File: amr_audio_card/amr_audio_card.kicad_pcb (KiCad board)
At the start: 2 copper layers, 68.8 x 106.7 mm, 3 parts, among them J1 Conn_Coaxial, J2 USB_A, U1 Bus_AMR

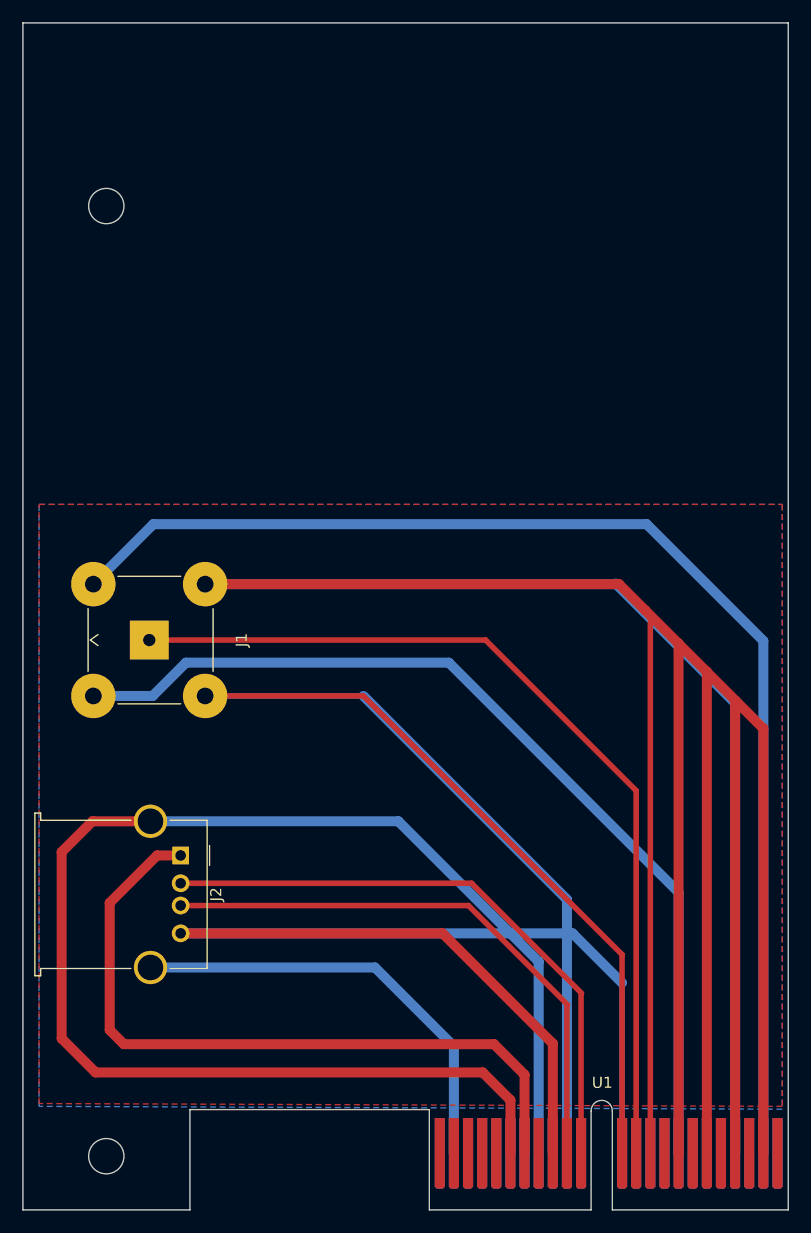
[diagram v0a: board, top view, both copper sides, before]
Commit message: yeah i don't need a bunch of empty space fabricated
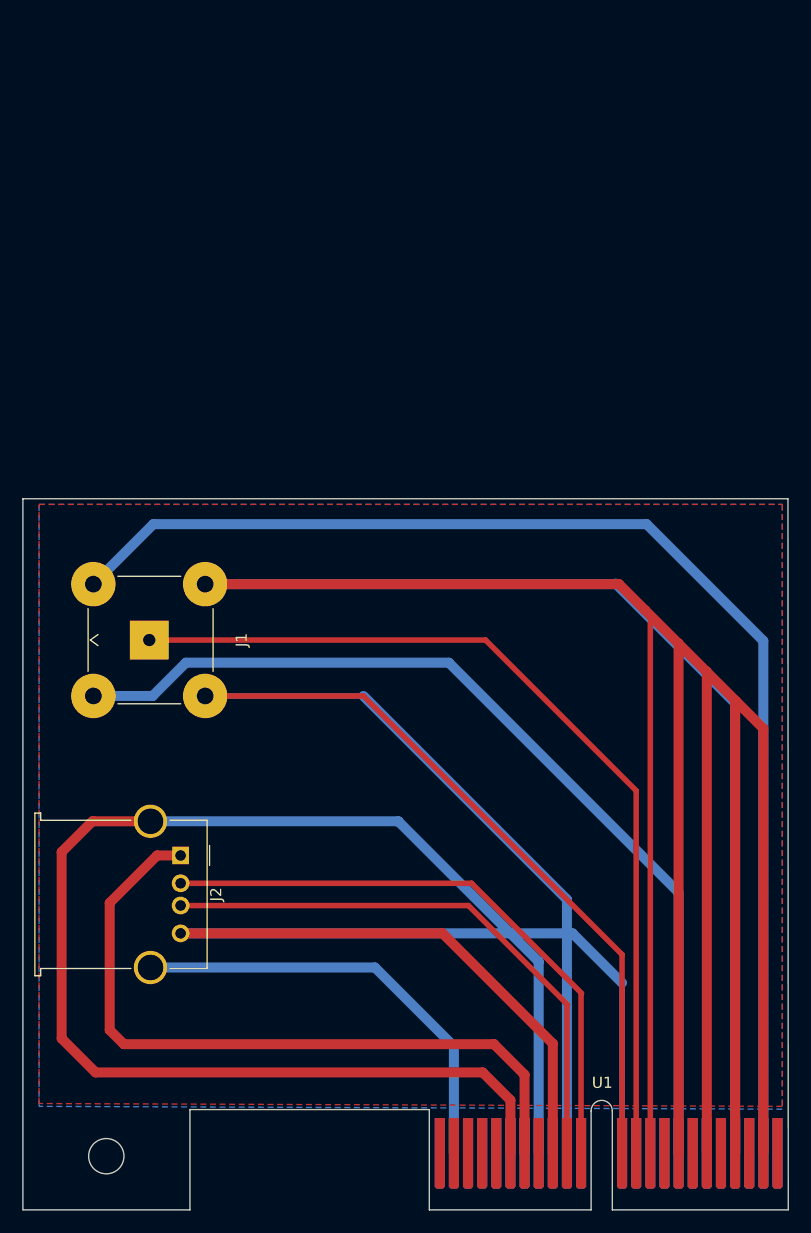
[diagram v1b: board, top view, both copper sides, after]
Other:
- board size 68.8 x 106.7 mm -> 68.8 x 63.9 mm
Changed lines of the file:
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@@
       (effects (font (size 1 1) (thickness 0.15)))
     )
-    (fp_line (start 0 0) (end 0 -106.68) (layer "Edge.Cuts") (width 0.12))
-    (fp_line (start 51.0667 -8.89) (end 51.0667 0) (layer "Edge.Cuts") (width 0.12))
+    (fp_line (start 0 0) (end 15.0114 0) (layer "Edge.Cuts") (width 0.12))
+    (fp_line (start 15.0114 -9.017) (end 36.5252 -9.017) (layer "Edge.Cuts") (width 0.12))
+    (fp_line (start 15.0114 0) (end 15.0114 -9.017) (layer "Edge.Cuts") (width 0.12))
+    (fp_line (start 51.0667 0) (end 36.5252 0) (layer "Edge.Cuts") (width 0.12))
+    (fp_line (start 52.9717 0) (end 68.7832 0) (layer "Edge.Cuts") (width 0.12))
     (fp_line (start 52.9717 -8.89) (end 52.9717 0) (layer "Edge.Cuts") (width 0.12))
     (fp_line (start 36.5252 0) (end 36.5252 -9.017) (layer "Edge.Cuts") (width 0.12))
-    (fp_line (start 68.7832 -106.68) (end 68.7832 0) (layer "Edge.Cuts") (width 0.12))
-    (fp_line (start 15.0114 0) (end 15.0114 -9.017) (layer "Edge.Cuts") (width 0.12))
-    (fp_line (start 15.0114 -9.017) (end 36.5252 -9.017) (layer "Edge.Cuts") (width 0.12))
-    (fp_line (start 52.9717 0) (end 68.7832 0) (layer "Edge.Cuts") (width 0.12))
-    (fp_line (start 51.0667 0) (end 36.5252 0) (layer "Edge.Cuts") (width 0.12))
-    (fp_line (start 0 -106.68) (end 68.7832 -106.68) (layer "Edge.Cuts") (width 0.12))
-    (fp_line (start 0 0) (end 15.0114 0) (layer "Edge.Cuts") (width 0.12))
+    (fp_line (start 51.0667 -8.89) (end 51.0667 0) (layer "Edge.Cuts") (width 0.12))
     (fp_arc (start 51.0667 -8.89) (mid 52.0192 -9.8425) (end 52.9717 -8.89) (layer "Edge.Cuts") (width 0.12))
-    (fp_circle (center 7.493 -90.2208) (end 9.0805 -90.2208) (layer "Edge.Cuts") (width 0.12) (fill none))
     (fp_circle (center 7.493 -4.826) (end 9.0805 -4.826) (layer "Edge.Cuts") (width 0.12) (fill none))
-    (fp_line (start 52.0192 0) (end 52.0192 -106.68) (layer "User.2") (width 0.12))
+    (fp_line (start 52.0192 0) (end 52.0192 -30.48) (layer "User.2") (width 0.12))
     (pad "A1" connect roundrect (at 37.465 -5.08) (size 0.9144 6.35) (layers "F.Cu" "F.Mask") (roundrect_rratio 0)
       (chamfer_ratio 0.2) (chamfer bottom_left bottom_right)
@@
     )
   )
+  (gr_line (start 161.544 99.06) (end 161.5682 162.975) (layer "Edge.Cuts") (width 0.1))
+  (gr_line (start 92.785 162.975) (end 92.785 99.06) (layer "Edge.Cuts") (width 0.1))
+  (gr_line (start 92.785 99.06) (end 161.544 99.06) (layer "Edge.Cuts") (width 0.1))
   (segment (start 147.903 157.895) (end 147.903 125.297) (width 0.5) (layer "F.Cu") (net 1))
   (segment (start 147.903 125.297) (end 134.366 111.76) (width 0.5) (layer "F.Cu") (net 1))
